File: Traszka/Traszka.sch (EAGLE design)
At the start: 12 parts, among them IC1 MEGA8-P, IC2 7818TV, X3 CRYSTALS-NOGND-HC49

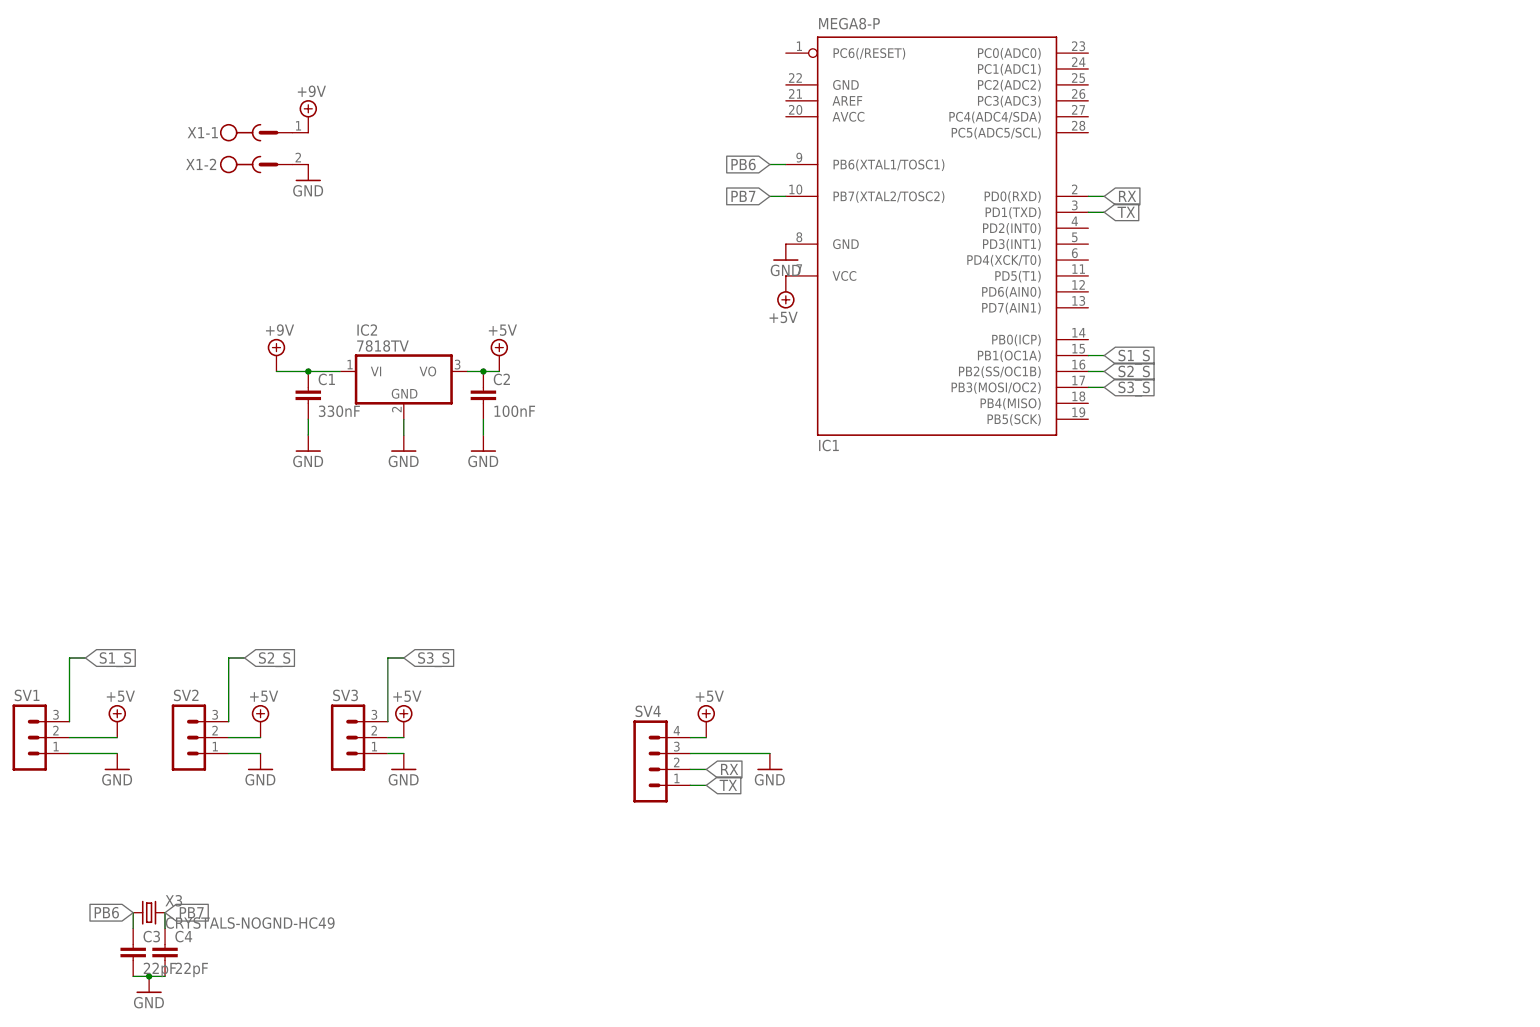
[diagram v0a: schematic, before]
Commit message: Final version
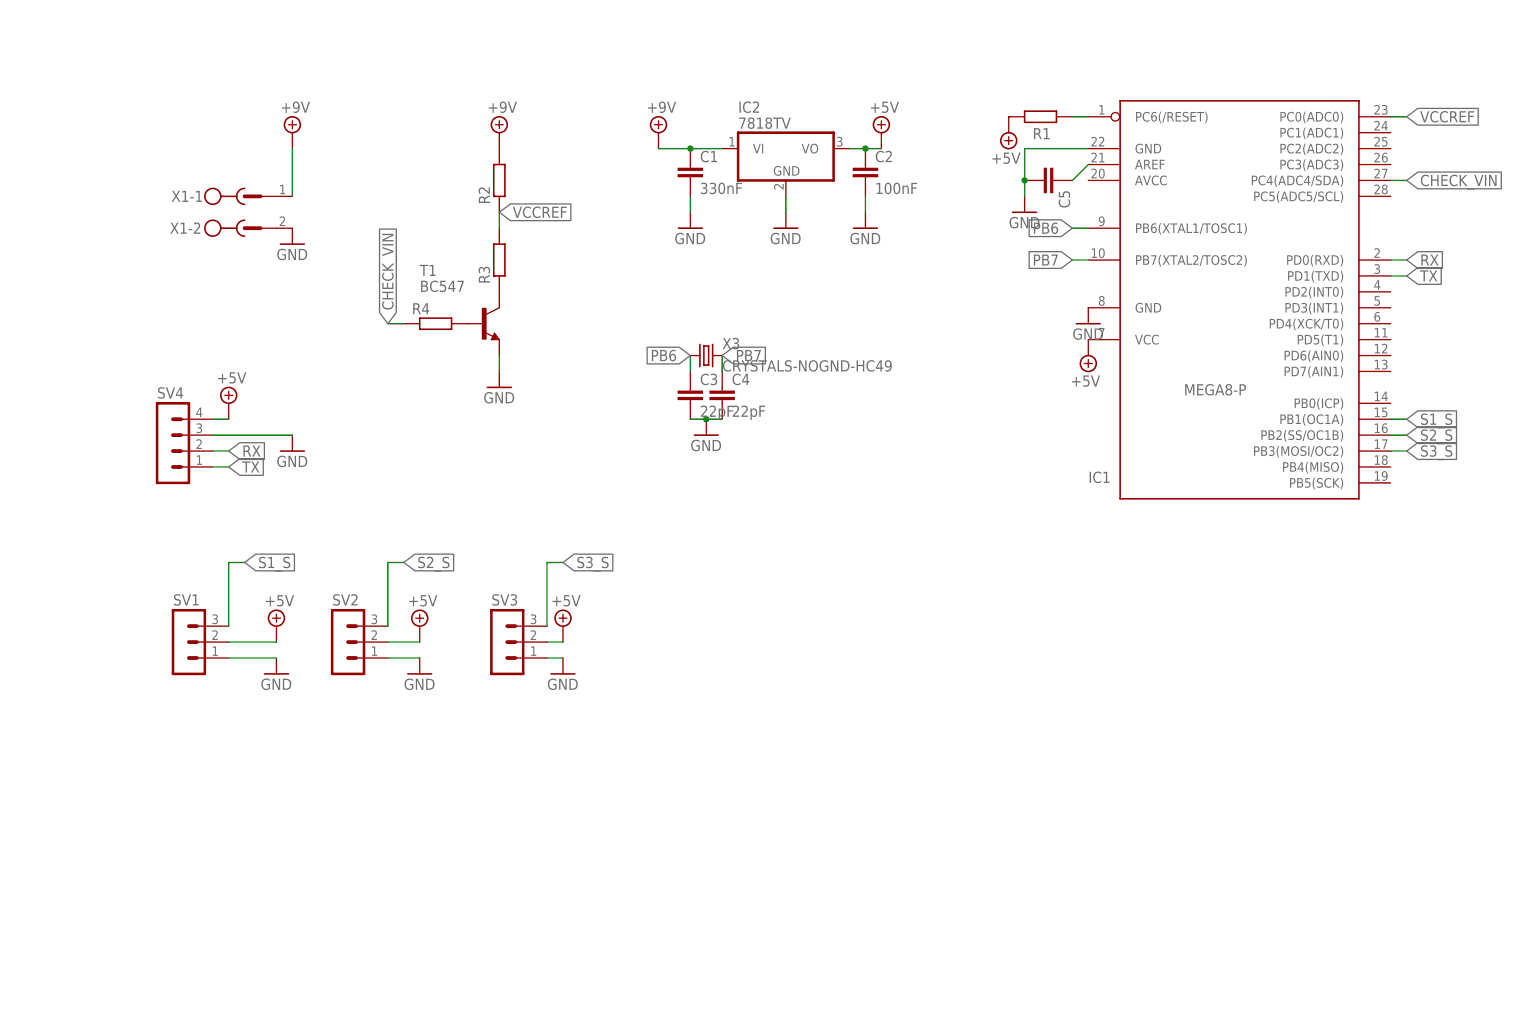
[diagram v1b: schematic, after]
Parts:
- added C5: (no value), rcl:C-EU050-024X044
- added R1, R2, R4: (no value), rcl:R-EU_0204/7
- added R3: (no value), rcl:R-EU_0204/5
- added T1: BC547, transistor:BC547
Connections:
- new net CHECK_VIN: IC1.PC4(ADC4/SDA), R4.1
- new net N$1: IC1.PC6(/RESET), R1.2
- new net N$2: C5.1, IC1.AREF
- new net N$3: R4.2, T1.B
- new net N$4: R3.1, T1.C
- new net VCCREF: IC1.PC0(ADC0), R2.1, R3.2
- net +5V: now also R1.1
- net +9V: now also R2.2
- net GND: now also C5.2, IC1.GND, T1.E
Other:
- moved on the sheet: C1, C2, C3, C4, IC1, IC2, SV1, SV2, SV3, SV4, X1-1, X1-2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
